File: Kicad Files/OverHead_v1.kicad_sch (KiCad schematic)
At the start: 12 parts, among them U1 ATMega2560

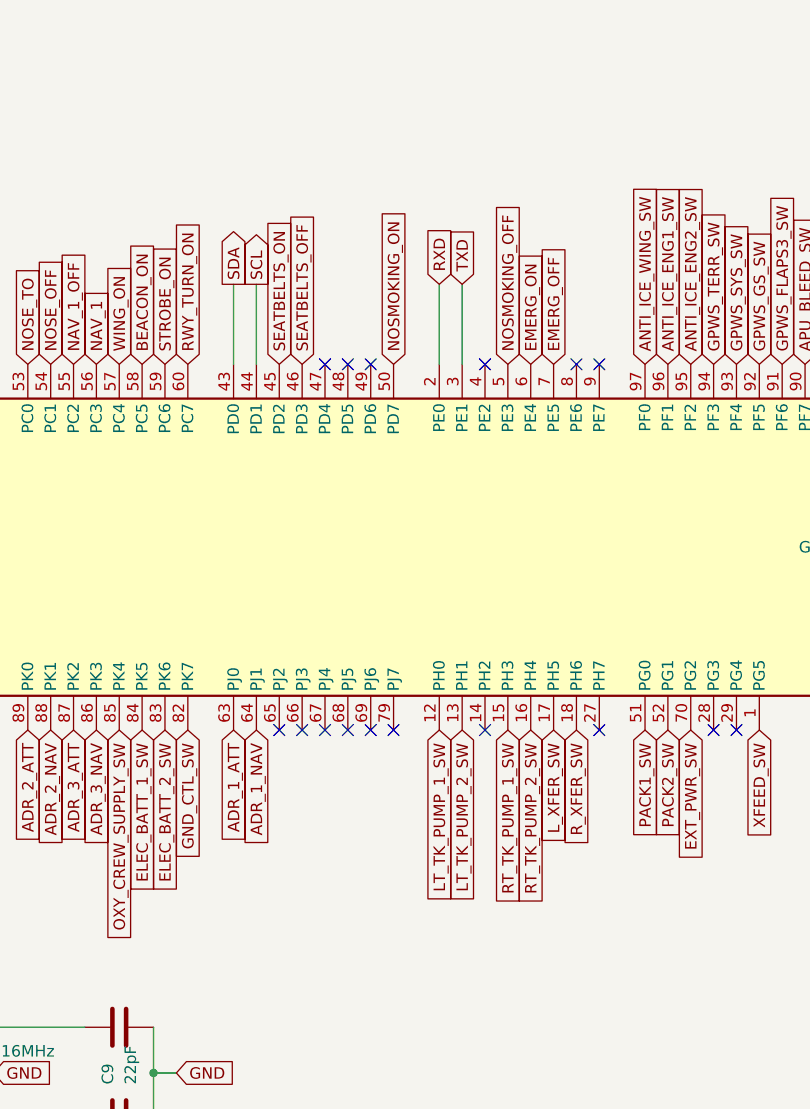
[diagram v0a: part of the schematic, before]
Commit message: New STL files for APU OVHD element, other coming in the next few weeks
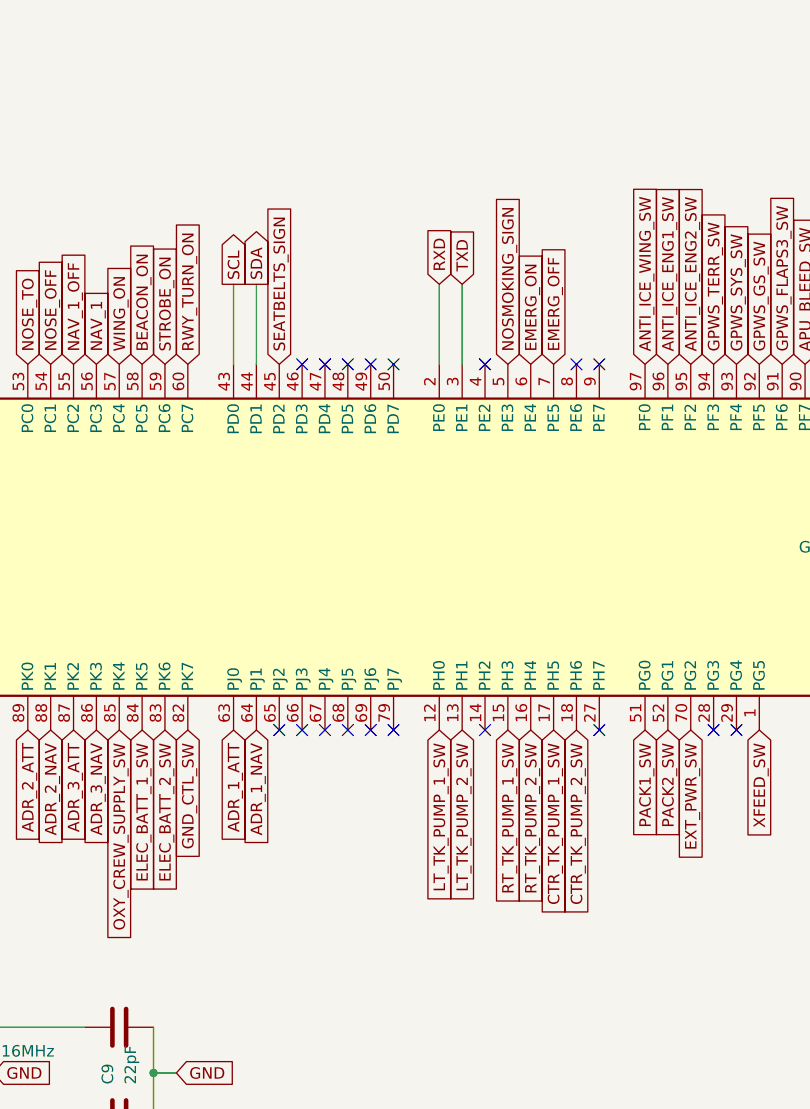
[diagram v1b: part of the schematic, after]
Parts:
- U1: footprint SFLibrary:TQFP100-0.5-14X14MM -> PCM_SFLibrary:TQFP100-0.5-14X14MM
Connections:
- net SCL: now also U1.43 (PD0); no longer U1.44 (PD1)
- net SDA: now also U1.44 (PD1); no longer U1.43 (PD0)
- net L_XFER_SW renamed CTR_TK_PUMP_1_SW
- net NOSMOKING_OFF renamed NOSMOKING_SIGN
- net NOSMOKING_ON: no longer names the net of U1.50 (PD7)
- net R_XFER_SW renamed CTR_TK_PUMP_2_SW
- net SEATBELTS_OFF: no longer names the net of U1.46 (PD3)
- net SEATBELTS_ON renamed SEATBELTS_SIGN
- no-connect marks 22 -> 24
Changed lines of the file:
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@@
 (kicad_sch
-	(version 20231120)
+	(version 20250114)
 	(generator "eeschema")
-	(generator_version "8.0")
+	(generator_version "9.0")
 	(paper "A4")
+	(text "DM13A Drivers"
+		(exclude_from_sim no)
+		(at 65.532 56.134 0)
+		(effects
+			(font
+				(size 1.27 1.27)
+			)
+		)
+	)
 	(junction
 		(at 33.02 76.2)
@@
 	)
 	(no_connect
+		(at 146.05 66.04)
+	)
+	(no_connect
 		(at 140.97 106.68)
 	)
 	(no_connect
+		(at 135.89 66.04)
+	)
+	(no_connect
 		(at 138.43 106.68)
 	)
@@
 		)
 	)
-	(text "DM13A Drivers"
-		(exclude_from_sim no)
-		(at 65.532 56.134 0)
-		(effects
-			(font
-				(size 1.27 1.27)
-			)
-		)
-	)
 	(global_label "ANTI_ICE_ENG2_SW"
 		(shape input)
@@
 		)
 	)
-	(global_label "SCL"
-		(shape output)
-		(at 130.81 57.15 90)
-		(fields_autoplaced yes)
-		(effects
-			(font
-				(size 1.27 1.27)
-			)
-			(justify left)
-		)
-		(property "Intersheetrefs" "${INTERSHEET_REFS}"
-			(at 130.81 50.6572 90)
-			(effects
-				(font
-					(size 1.27 1.27)
-				)
-				(justify left)
-				(hide yes)
-			)
-		)
-	)
 	(global_label "ANTI_ICE_ENG1_SW"
 		(shape input)
@@
 		)
 	)
-	(global_label "L_XFER_SW"
+	(global_label "CTR_TK_PUMP_1_SW"
 		(shape input)
 		(at 163.83 106.68 270)
@@
 		)
 		(property "Intersheetrefs" "${INTERSHEET_REFS}"
-			(at 163.83 120.0065 90)
+			(at 163.83 128.4731 90)
 			(effects
 				(font
@@
 		)
 	)
+	(global_label "NOSMOKING_SIGN"
+		(shape input)
+		(at 158.75 66.04 90)
+		(fields_autoplaced yes)
+		(effects
+			(font
+				(size 1.27 1.27)
+			)
+			(justify left)
+		)
+		(property "Intersheetrefs" "${INTERSHEET_REFS}"
+			(at 158.75 46.5447 90)
+			(effects
+				(font
+					(size 1.27 1.27)
+				)
+				(justify left)
+				(hide yes)
+			)
+		)
+	)
 	(global_label "LCH2"
 		(shape input)
@@
 		)
 	)
-	(global_label "NOSMOKING_OFF"
-		(shape input)
-		(at 158.75 66.04 90)
+	(global_label "SCL"
+		(shape output)
+		(at 128.27 57.15 90)
 		(fields_autoplaced yes)
 		(effects
@@
 		)
 		(property "Intersheetrefs" "${INTERSHEET_REFS}"
-			(at 158.75 47.4518 90)
+			(at 128.27 50.6572 90)
 			(effects
 				(font
@@
 		)
 	)
+	(global_label "SDA"
+		(shape output)
+		(at 130.81 57.15 90)
+		(fields_autoplaced yes)
+		(effects
+			(font
+				(size 1.27 1.27)
+			)
+			(justify left)
+		)
+		(property "Intersheetrefs" "${INTERSHEET_REFS}"
+			(at 130.81 50.5967 90)
+			(effects
+				(font
+					(size 1.27 1.27)
+				)
+				(justify left)
+				(hide yes)
+			)
+		)
+	)
 	(global_label "GPWS_SYS_SW"
 		(shape input)
@@
 		)
 	)
-	(global_label "NOSMOKING_ON"
-		(shape input)
-		(at 146.05 66.04 90)
-		(fields_autoplaced yes)
-		(effects
-			(font
-				(size 1.27 1.27)
-			)
-			(justify left)
-		)
-		(property "Intersheetrefs" "${INTERSHEET_REFS}"
-			(at 146.05 48.2985 90)
-			(effects
-				(font
-					(size 1.27 1.27)
-				)
-				(justify left)
-				(hide yes)
-			)
-		)
-	)
 	(global_label "STROBE_ON"
 		(shape input)
@@
 		)
 	)
-	(global_label "SDA"
-		(shape output)
-		(at 128.27 57.15 90)
-		(fields_autoplaced yes)
-		(effects
-			(font
-				(size 1.27 1.27)
-			)
-			(justify left)
-		)
-		(property "Intersheetrefs" "${INTERSHEET_REFS}"
-			(at 128.27 50.5967 90)
-			(effects
-				(font
-					(size 1.27 1.27)
-				)
-				(justify left)
-				(hide yes)
-			)
-		)
-	)
 	(global_label "ADR_1_NAV"
 		(shape input)
@@
 		)
 	)
-	(global_label "SEATBELTS_ON"
+	(global_label "SEATBELTS_SIGN"
 		(shape input)
 		(at 133.35 66.04 90)
@@
 		)
 		(property "Intersheetrefs" "${INTERSHEET_REFS}"
-			(at 133.35 49.3873 90)
-			(effects
-				(font
-					(size 1.27 1.27)
-				)
-				(justify left)
-				(hide yes)
-			)
-		)
-	)
-	(global_label "SEATBELTS_OFF"
-		(shape input)
-		(at 135.89 66.04 90)
-		(fields_autoplaced yes)
-		(effects
-			(font
-				(size 1.27 1.27)
-			)
-			(justify left)
-		)
-		(property "Intersheetrefs" "${INTERSHEET_REFS}"
-			(at 135.89 48.5406 90)
+			(at 133.35 47.6335 90)
 			(effects
 				(font
@@
 		)
 	)
-	(global_label "R_XFER_SW"
+	(global_label "CTR_TK_PUMP_2_SW"
 		(shape input)
 		(at 166.37 106.68 270)
@@
 		)
 		(property "Intersheetrefs" "${INTERSHEET_REFS}"
-			(at 166.37 120.2484 90)
+			(at 166.37 128.4731 90)
 			(effects
 				(font
@@
 			)
 		)
-		(property "Footprint" "SFLibrary:TQFP100-0.5-14X14MM"
+		(property "Footprint" "PCM_SFLibrary:TQFP100-0.5-14X14MM"
 			(at 125.73 86.36 0)
 			(effects
@@
 		(at 0 215.9)
 		(size 297.18 187.96)
+		(exclude_from_sim no)
+		(in_bom yes)
+		(on_board yes)
+		(dnp no)
 		(fields_autoplaced yes)
 		(stroke
@@
 		(at 838.2 0)
 		(size 255.27 209.55)
+		(exclude_from_sim no)
+		(in_bom yes)
+		(on_board yes)
+		(dnp no)
 		(fields_autoplaced yes)
 		(stroke
@@
 		(at 0 412.75)
 		(size 298.45 176.53)
+		(exclude_from_sim no)
+		(in_bom yes)
+		(on_board yes)
+		(dnp no)
 		(fields_autoplaced yes)
 		(stroke
@@
 		(at 572.77 412.75)
 		(size 256.54 176.53)
+		(exclude_from_sim no)
+		(in_bom yes)
+		(on_board yes)
+		(dnp no)
 		(fields_autoplaced yes)
 		(stroke
@@
 		(at 571.5 215.9)
 		(size 257.81 187.96)
+		(exclude_from_sim no)
+		(in_bom yes)
+		(on_board yes)
+		(dnp no)
 		(fields_autoplaced yes)
 		(stroke
@@
 		(at 836.93 412.75)
 		(size 257.81 176.53)
+		(exclude_from_sim no)
+		(in_bom yes)
+		(on_board yes)
+		(dnp no)
 		(fields_autoplaced yes)
 		(stroke
@@
 		(at 304.8 412.75)
 		(size 262.89 176.53)
+		(exclude_from_sim no)
+		(in_bom yes)
+		(on_board yes)
+		(dnp no)
 		(fields_autoplaced yes)
 		(stroke
@@
 		(at 1103.63 0)
 		(size 236.22 208.28)
+		(exclude_from_sim no)
+		(in_bom yes)
+		(on_board yes)
+		(dnp no)
 		(fields_autoplaced yes)
 		(stroke
@@
 		(at 1103.63 215.9)
 		(size 236.22 187.96)
+		(exclude_from_sim no)
+		(in_bom yes)
+		(on_board yes)
+		(dnp no)
 		(fields_autoplaced yes)
 		(stroke
@@
 		(at 304.8 0)
 		(size 262.89 209.55)
+		(exclude_from_sim no)
+		(in_bom yes)
+		(on_board yes)
+		(dnp no)
 		(fields_autoplaced yes)
 		(stroke
@@
 		(at 0 596.9)
 		(size 297.18 168.91)
+		(exclude_from_sim no)
+		(in_bom yes)
+		(on_board yes)
+		(dnp no)
 		(fields_autoplaced yes)
 		(stroke
@@
 		(at 838.2 215.9)
 		(size 255.27 187.96)
+		(exclude_from_sim no)
+		(in_bom yes)
+		(on_board yes)
+		(dnp no)
 		(fields_autoplaced yes)
 		(stroke
@@
 		(at 304.8 215.9)
 		(size 262.89 187.96)
+		(exclude_from_sim no)
+		(in_bom yes)
+		(on_board yes)
+		(dnp no)
 		(fields_autoplaced yes)
 		(stroke
@@
 		(at 571.5 0)
 		(size 257.81 209.55)
+		(exclude_from_sim no)
+		(in_bom yes)
+		(on_board yes)
+		(dnp no)
 		(fields_autoplaced yes)
 		(stroke
@@
 		)
 	)
+	(embedded_fonts no)
 )
